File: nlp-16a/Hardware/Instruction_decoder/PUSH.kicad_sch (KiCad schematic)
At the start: 7 parts

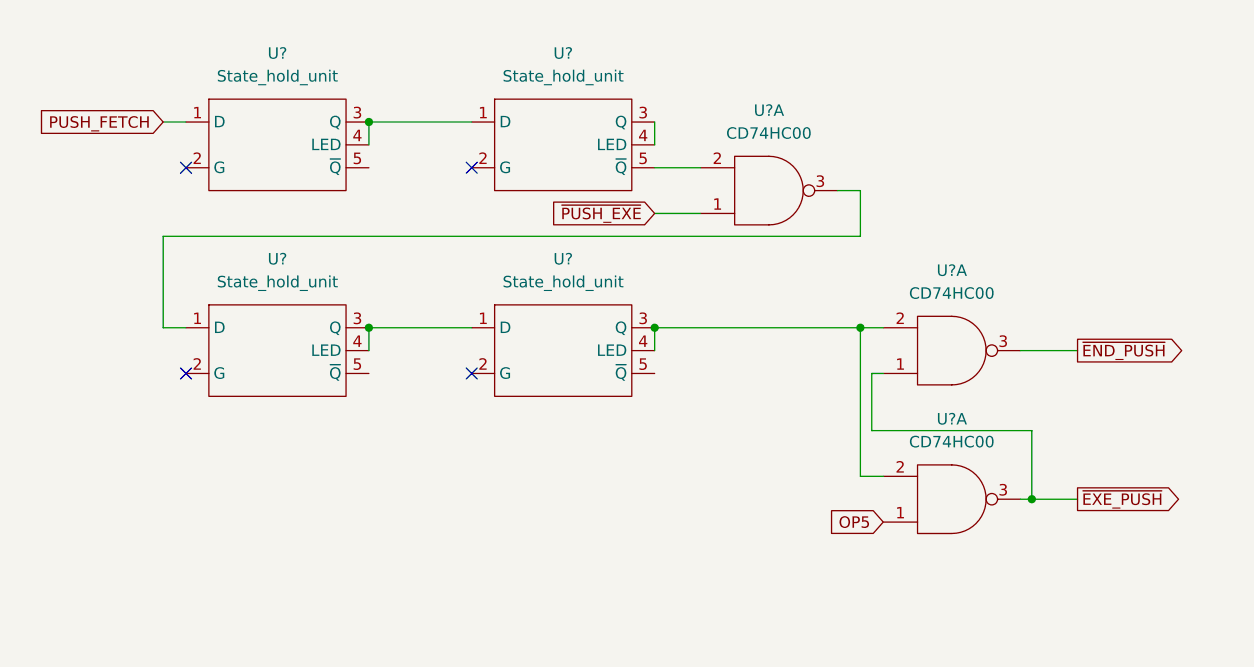
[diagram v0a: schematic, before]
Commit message: 命令デコーダ ロジック部の設計だいたい完了git statusgit statusやったぜ
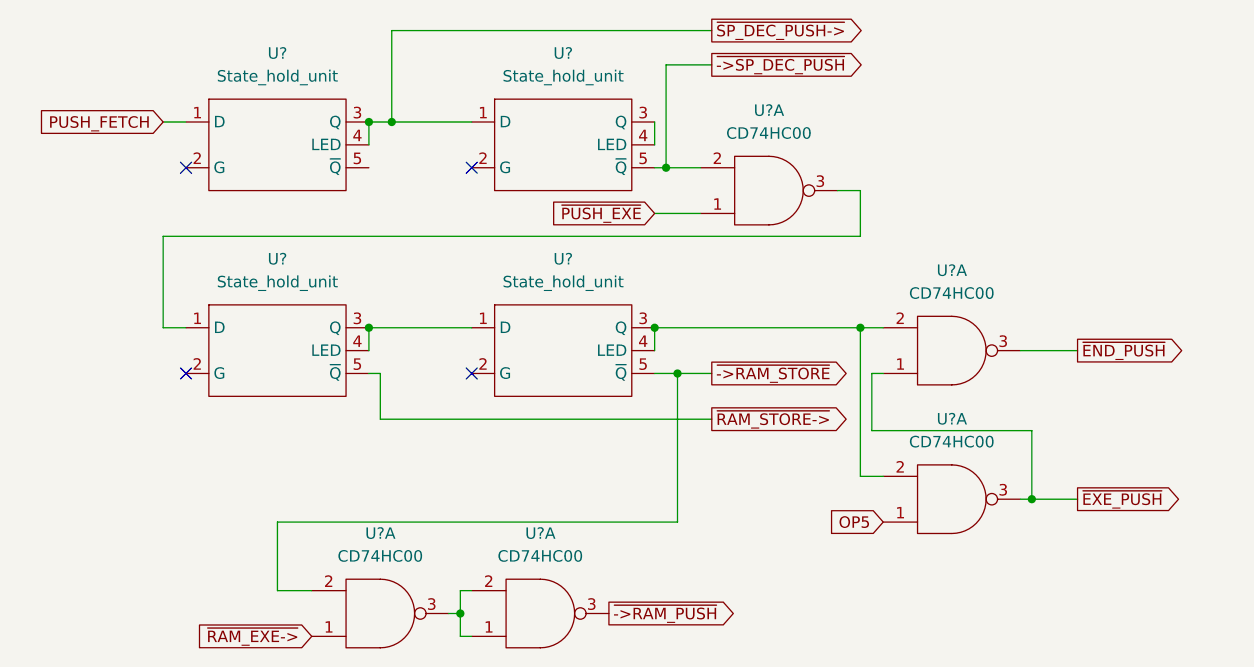
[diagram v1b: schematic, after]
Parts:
- added U? (x2): CD74HC00, Package_DIP:DIP-14_W7.62mm, symbol CD74HCXX:CD74HC00
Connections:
- net GND: now also U?.7 (GND), U?.7 (GND)
- net VCC: now also U?.14 (VCC), U?.14 (VCC)
- net ~{SP_DEC_PUSH->}: now reaches U?.1 (D), U?.3 (Q), U?.4 (LED)
- net ~{->SP_DEC_PUSH}: now reaches U?.2, U?.5 (~{Q})
- net ~{->RAM_STORE}: now reaches U?.5 (~{Q})
- net ~{->RAM_STORE}: now also U?.2
- net ~{RAM_STORE->}: now reaches U?.5 (~{Q})
- new net: U?.1, U?.2, U?.3
- new net ~{->RAM_PUSH}: U?.3
- new net ~{RAM_EXE->}: U?.1
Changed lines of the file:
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@@
   (junction (at 125.73 69.85) (diameter 0) (color 0 0 0 0)
   )
+  (junction (at 158.75 52.07) (diameter 0) (color 0 0 0 0)
+  )
   (junction (at 199.39 88.9) (diameter 0) (color 0 0 0 0)
+  )
+  (junction (at 160.02 74.93) (diameter 0) (color 0 0 0 0)
+  )
+  (junction (at 128.27 46.99) (diameter 0) (color 0 0 0 0)
+  )
+  (junction (at 135.89 101.6) (diameter 0) (color 0 0 0 0)
   )
   (junction (at 157.48 69.85) (diameter 0) (color 0 0 0 0)
@@
   (no_connect (at 137.16 74.93))
   (no_connect (at 105.41 74.93))
+  (wire (pts (xy 135.89 104.14) (xy 135.89 101.6))
+    (stroke (width 0) (type default) (color 0 0 0 0))
+  )
+  (wire (pts (xy 115.57 99.06) (xy 115.57 91.44))
+    (stroke (width 0) (type default) (color 0 0 0 0))
+  )
+  (wire (pts (xy 135.89 101.6) (xy 135.89 99.06))
+    (stroke (width 0) (type default) (color 0 0 0 0))
+  )
   (wire (pts (xy 199.39 88.9) (xy 198.12 88.9))
     (stroke (width 0) (type default) (color 0 0 0 0))
   )
+  (wire (pts (xy 134.62 101.6) (xy 135.89 101.6))
+    (stroke (width 0) (type default) (color 0 0 0 0))
+  )
   (wire (pts (xy 102.87 59.69) (xy 180.34 59.69))
     (stroke (width 0) (type default) (color 0 0 0 0))
   )
+  (wire (pts (xy 157.48 52.07) (xy 158.75 52.07))
+    (stroke (width 0) (type default) (color 0 0 0 0))
+  )
+  (wire (pts (xy 160.02 91.44) (xy 160.02 74.93))
+    (stroke (width 0) (type default) (color 0 0 0 0))
+  )
+  (wire (pts (xy 115.57 91.44) (xy 160.02 91.44))
+    (stroke (width 0) (type default) (color 0 0 0 0))
+  )
   (wire (pts (xy 182.88 69.85) (xy 180.34 69.85))
     (stroke (width 0) (type default) (color 0 0 0 0))
   )
+  (wire (pts (xy 128.27 36.83) (xy 128.27 46.99))
+    (stroke (width 0) (type default) (color 0 0 0 0))
+  )
   (wire (pts (xy 180.34 69.85) (xy 180.34 86.36))
     (stroke (width 0) (type default) (color 0 0 0 0))
   )
+  (wire (pts (xy 128.27 46.99) (xy 137.16 46.99))
+    (stroke (width 0) (type default) (color 0 0 0 0))
+  )
+  (wire (pts (xy 158.75 52.07) (xy 162.56 52.07))
+    (stroke (width 0) (type default) (color 0 0 0 0))
+  )
   (wire (pts (xy 105.41 69.85) (xy 102.87 69.85))
     (stroke (width 0) (type default) (color 0 0 0 0))
@@
     (stroke (width 0) (type default) (color 0 0 0 0))
   )
+  (wire (pts (xy 160.02 74.93) (xy 163.83 74.93))
+    (stroke (width 0) (type default) (color 0 0 0 0))
+  )
+  (wire (pts (xy 125.73 46.99) (xy 128.27 46.99))
+    (stroke (width 0) (type default) (color 0 0 0 0))
+  )
+  (wire (pts (xy 158.75 40.64) (xy 158.75 52.07))
+    (stroke (width 0) (type default) (color 0 0 0 0))
+  )
   (wire (pts (xy 180.34 54.61) (xy 177.8 54.61))
     (stroke (width 0) (type default) (color 0 0 0 0))
@@
     (stroke (width 0) (type default) (color 0 0 0 0))
   )
+  (wire (pts (xy 163.83 80.01) (xy 127 80.01))
+    (stroke (width 0) (type default) (color 0 0 0 0))
+  )
   (wire (pts (xy 157.48 57.15) (xy 162.56 57.15))
     (stroke (width 0) (type default) (color 0 0 0 0))
   )
-  (wire (pts (xy 157.48 52.07) (xy 162.56 52.07))
+  (wire (pts (xy 135.89 99.06) (xy 137.16 99.06))
+    (stroke (width 0) (type default) (color 0 0 0 0))
+  )
+  (wire (pts (xy 119.38 99.06) (xy 115.57 99.06))
+    (stroke (width 0) (type default) (color 0 0 0 0))
+  )
+  (wire (pts (xy 157.48 74.93) (xy 160.02 74.93))
     (stroke (width 0) (type default) (color 0 0 0 0))
   )
@@
     (stroke (width 0) (type default) (color 0 0 0 0))
   )
+  (wire (pts (xy 137.16 104.14) (xy 135.89 104.14))
+    (stroke (width 0) (type default) (color 0 0 0 0))
+  )
   (wire (pts (xy 180.34 86.36) (xy 182.88 86.36))
     (stroke (width 0) (type default) (color 0 0 0 0))
   )
-  (wire (pts (xy 125.73 46.99) (xy 137.16 46.99))
-    (stroke (width 0) (type default) (color 0 0 0 0))
-  )
   (wire (pts (xy 102.87 69.85) (xy 102.87 59.69))
     (stroke (width 0) (type default) (color 0 0 0 0))
   )
+  (wire (pts (xy 127 74.93) (xy 125.73 74.93))
+    (stroke (width 0) (type default) (color 0 0 0 0))
+  )
+  (wire (pts (xy 163.83 40.64) (xy 158.75 40.64))
+    (stroke (width 0) (type default) (color 0 0 0 0))
+  )
   (wire (pts (xy 180.34 59.69) (xy 180.34 54.61))
     (stroke (width 0) (type default) (color 0 0 0 0))
@@
     (stroke (width 0) (type default) (color 0 0 0 0))
   )
+  (wire (pts (xy 163.83 36.83) (xy 128.27 36.83))
+    (stroke (width 0) (type default) (color 0 0 0 0))
+  )
+  (wire (pts (xy 127 80.01) (xy 127 74.93))
+    (stroke (width 0) (type default) (color 0 0 0 0))
+  )
   (global_label "~{EXE_PUSH}" (shape output) (at 204.47 88.9 0) (fields_autoplaced)
     (effects (font (size 1.27 1.27)) (justify left))
@@
     )
   )
+  (global_label "~{RAM_EXE->}" (shape input) (at 119.38 104.14 180) (fields_autoplaced)
+    (effects (font (size 1.27 1.27)) (justify right))
+    (property "Intersheet References" "${INTERSHEET_REFS}" (id 0) (at 105.5369 104.0606 0)
+      (effects (font (size 1.27 1.27)) (justify right) hide)
+    )
+  )
+  (global_label "~{->RAM_PUSH}" (shape output) (at 152.4 101.6 0) (fields_autoplaced)
+    (effects (font (size 1.27 1.27)) (justify left))
+    (property "Intersheet References" "${INTERSHEET_REFS}" (id 0) (at 167.876 101.5206 0)
+      (effects (font (size 1.27 1.27)) (justify left) hide)
+    )
+  )
+  (global_label "~{->SP_DEC_PUSH}" (shape output) (at 163.83 40.64 0) (fields_autoplaced)
+    (effects (font (size 1.27 1.27)) (justify left))
+    (property "Intersheet References" "${INTERSHEET_REFS}" (id 0) (at 182.6321 40.5606 0)
+      (effects (font (size 1.27 1.27)) (justify left) hide)
+    )
+  )
   (global_label "OP5" (shape input) (at 182.88 91.44 180) (fields_autoplaced)
     (effects (font (size 1.27 1.27)) (justify right))
@@
     )
   )
+  (global_label "~{SP_DEC_PUSH->}" (shape output) (at 163.83 36.83 0) (fields_autoplaced)
+    (effects (font (size 1.27 1.27)) (justify left))
+    (property "Intersheet References" "${INTERSHEET_REFS}" (id 0) (at 182.6321 36.7506 0)
+      (effects (font (size 1.27 1.27)) (justify left) hide)
+    )
+  )
   (global_label "PUSH_FETCH" (shape input) (at 102.87 46.99 180) (fields_autoplaced)
     (effects (font (size 1.27 1.27)) (justify right))
@@
     )
   )
+  (global_label "~{RAM_STORE->}" (shape output) (at 163.83 80.01 0) (fields_autoplaced)
+    (effects (font (size 1.27 1.27)) (justify left))
+    (property "Intersheet References" "${INTERSHEET_REFS}" (id 0) (at 180.0921 79.9306 0)
+      (effects (font (size 1.27 1.27)) (justify left) hide)
+    )
+  )
   (global_label "~{END_PUSH}" (shape output) (at 204.47 72.39 0) (fields_autoplaced)
     (effects (font (size 1.27 1.27)) (justify left))
@@
       (effects (font (size 1.27 1.27)) (justify left) hide)
     )
+  )
+  (global_label "~{->RAM_STORE}" (shape output) (at 163.83 74.93 0) (fields_autoplaced)
+    (effects (font (size 1.27 1.27)) (justify left))
+    (property "Intersheet References" "${INTERSHEET_REFS}" (id 0) (at 180.0921 74.8506 0)
+      (effects (font (size 1.27 1.27)) (justify left) hide)
+    )
+  )
+  (symbol (lib_id "CD74HCXX:CD74HC00") (at 144.78 101.6 0) (mirror x) (unit 1)
+    (in_bom yes) (on_board yes)
+    (property "Reference" "U?" (id 0) (at 144.78 92.71 0))
+    (property "Value" "CD74HC00" (id 1) (at 144.78 95.25 0))
+    (property "Footprint" "Package_DIP:DIP-14_W7.62mm" (id 2) (at 144.78 107.95 0)
+      (effects (font (size 1.27 1.27)) hide)
+    )
+    (property "Datasheet" "" (id 3) (at 139.7 101.6 0))
+    (pin "14")
+    (pin "7")
+    (pin "1")
+    (pin "2")
+    (pin "3")
+    (pin "4")
+    (pin "5")
+    (pin "6")
+    (pin "10")
+    (pin "8")
+    (pin "9")
+    (pin "11")
+    (pin "12")
+    (pin "13")
   )
   (symbol (lib_id "CD74HCXX:CD74HC00") (at 190.5 72.39 0) (mirror x) (unit 1)
@@
     (pin "14")
     (pin "7")
+    (pin "1")
+    (pin "2")
+    (pin "3")
+    (pin "4")
+    (pin "5")
+    (pin "6")
+    (pin "10")
+    (pin "8")
+    (pin "9")
+    (pin "11")
+    (pin "12")
+    (pin "13")
+  )
+  (symbol (lib_id "CD74HCXX:CD74HC00") (at 127 101.6 0) (mirror x) (unit 1)
+    (in_bom yes) (on_board yes)
+    (property "Reference" "U?" (id 0) (at 127 92.71 0))
+    (property "Value" "CD74HC00" (id 1) (at 127 95.25 0))
+    (property "Footprint" "Package_DIP:DIP-14_W7.62mm" (id 2) (at 127 107.95 0)
+      (effects (font (size 1.27 1.27)) hide)
+    )
+    (property "Datasheet" "" (id 3) (at 121.92 101.6 0))
+    (pin "14")
+    (pin "7")
